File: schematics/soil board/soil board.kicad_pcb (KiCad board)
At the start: 2 copper layers, 30 x 114 mm, 17 parts, among them J1 AVR-ISP-6, J2 1989748, J3 1989748, J4 1989748, U1 ATtiny841-SS, U3 MCP9700Ax-ETT

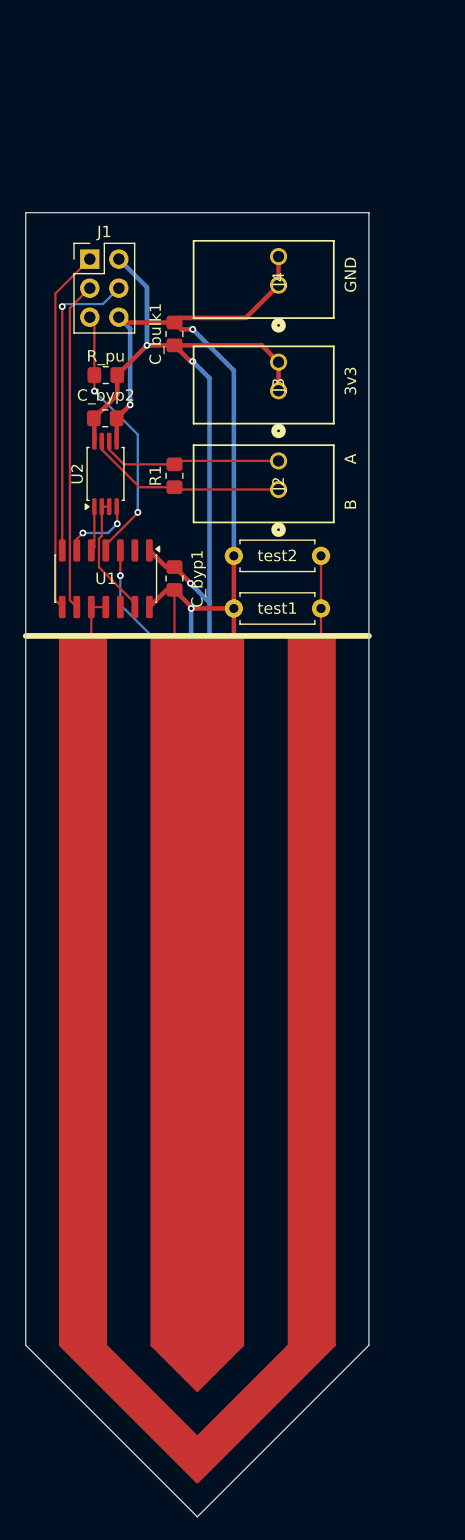
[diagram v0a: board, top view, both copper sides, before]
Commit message: Interface for temp sensor and soil moisture sensor
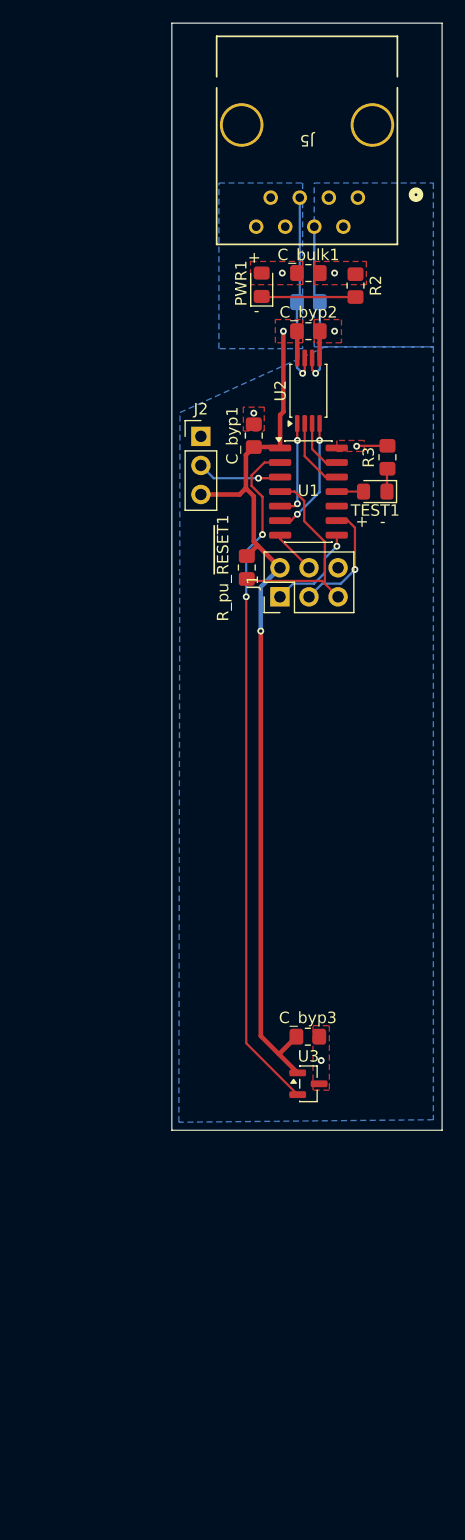
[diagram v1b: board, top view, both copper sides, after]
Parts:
- removed Elecctrodes1: C, soil_cap:Untitled
- removed J3, J4: 1989748, footprints:CONN_1989748_PXC
- removed R_pu: 10k, Resistor_SMD:R_0805_2012Metric_Pad1.20x1.40mm_HandSolder
- removed test1, test2: R_US, Resistor_THT:R_Axial_DIN0207_L6.3mm_D2.5mm_P7.62mm_Horizontal
- added J5: 54602-908LF, 54602_908LF_footprints:CONN8_2-908LF_AMP, F.Cu at (97.0, 74.7)
- added PWR1: LED, LED_SMD:LED_0805_2012Metric_Pad1.15x1.40mm_HandSolder, F.Cu at (88.6, 82.3)
- added R2: 56, Resistor_SMD:R_0805_2012Metric_Pad1.20x1.40mm_HandSolder, F.Cu at (96.8, 82.4)
- added R3: 56, Resistor_SMD:R_0805_2012Metric_Pad1.20x1.40mm_HandSolder, F.Cu at (99.6, 97.4)
- added R_pu_~{RESET}1: 10k, Resistor_SMD:R_0805_2012Metric_Pad1.20x1.40mm_HandSolder, F.Cu at (87.3, 107.0)
- added TEST1: LED, LED_SMD:LED_0805_2012Metric_Pad1.15x1.40mm_HandSolder, F.Cu at (98.6, 100.4)
- C_byp3, U3: moved to F.Cu
- J2: value 1989748 -> Conn_01x03_Pin; footprint footprints:CONN_1989748_PXC -> Connector_PinHeader_2.54mm:PinHeader_1x03_P2.54mm_Vertical
- R1: value R_US -> 120; moved to B.Cu
- moved J1 33.9 mm to (90.2, 109.6), turned to 90 degrees
- moved C_byp2 19.3 mm to (92.7, 86.4)
- moved U1 19.3 mm to (92.7, 100.4), turned to 0 degrees
- moved R1 19.2 mm to (92.7, 83.8), turned to 0 degrees
- moved U2 19.2 mm to (92.7, 91.6)
- moved C_byp1 14.3 mm to (87.9, 95.5), turned to 90 degrees
- moved C_bulk1 12.9 mm to (92.7, 81.3), turned to 0 degrees
- moved C_byp3 12.8 mm to (92.7, 148.0), turned to 0 degrees
- moved U3 12.7 mm to (92.7, 152.1), turned to 0 degrees
- moved J2 8.23 mm to (83.3, 95.6), turned to 0 degrees
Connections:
- J2 pad 1: Net-(U2-B) -> GND
- J2 pad 2: Net-(U2-A) -> ADC_10_moisture
- U1 pad 10: CAP_CHARGE -> unconnected-(U1-PA3-Pad10)
- U1 pad 11: CAP_CHARGE -> Net-(TEST1-A)
- U1 pad 12: unconnected-(U1-PA1-Pad12) -> /RE
- U1 pad 13: DE/~{RE} -> DE
- U1 pad 2: unconnected-(U1-XTAL1/PB0-Pad2) -> ADC_11_temp
- U1 pad 3: ADC_11_temp -> ADC_10_moisture
- U2 pad 2: DE/~{RE} -> /RE
- U2 pad 3: DE/~{RE} -> DE
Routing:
- net GND: track 168.3 -> 5.08 mm, vias 3 -> 5
- net MISO: track 31.9 -> 8.53 mm, vias 0 -> 1
- net MOSI: track 27.2 -> 4.22 mm, vias 1 -> 0
- net SCK: track 28.8 -> 10.5 mm, vias 0 -> 1
- net +3.3V: track 99.7 -> 81.6 mm
- net ADC_11_temp: track 41.8 -> 59.9 mm, vias 1 -> 2
- net CAP_CHARGE: track 13.1 -> 0.00 mm
- net DE/~{RE}: track 10.8 -> 0.00 mm
- net Net-(PWR1-K): track 0.00 -> 8.22 mm
- net ADC_10_moisture: track 0.00 -> 7.43 mm, vias 0 -> 1
- net /RE: track 0.00 -> 6.44 mm
- net ~{RESET}: track 24.6 -> 19.1 mm, vias 2 -> 0
- net DE: track 0.00 -> 4.87 mm
- net TXD0_ALT: track 6.60 -> 10.6 mm
- net RXD0_ALT: track 5.19 -> 8.62 mm, vias 0 -> 2
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- added copper zone on B.Cu, net +3.3V
- added copper zone on F.Cu, net +3.3V
- added copper zone on B.Cu, net GND
- added copper zone on F.Cu, net GND
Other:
- board size 30 x 114 mm -> 23.6 x 96.8 mm
- board text added: "+"
- board text added: "-"
- board text removed: "3v3"
- board text removed: "A"
- board text removed: "B"
- board text removed: "GND"
